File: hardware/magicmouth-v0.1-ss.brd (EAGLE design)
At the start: 100 x 80 mm, 34 parts, among them IC1 LM386N, IC2 ATMEGA328P_PDIP, Q1 16Mhz, U1 ARDUINOR3-NOIOREF-NOTEXT

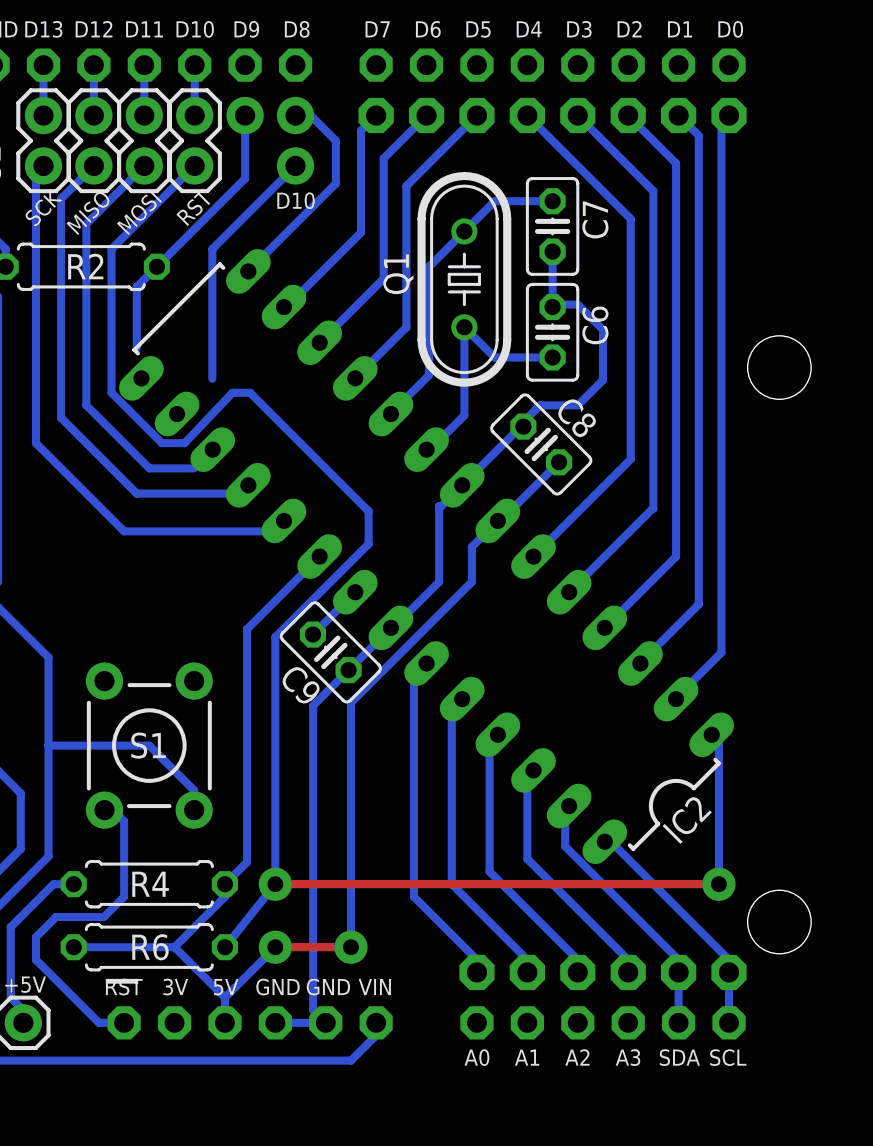
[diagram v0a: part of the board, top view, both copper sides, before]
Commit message: trace corrections
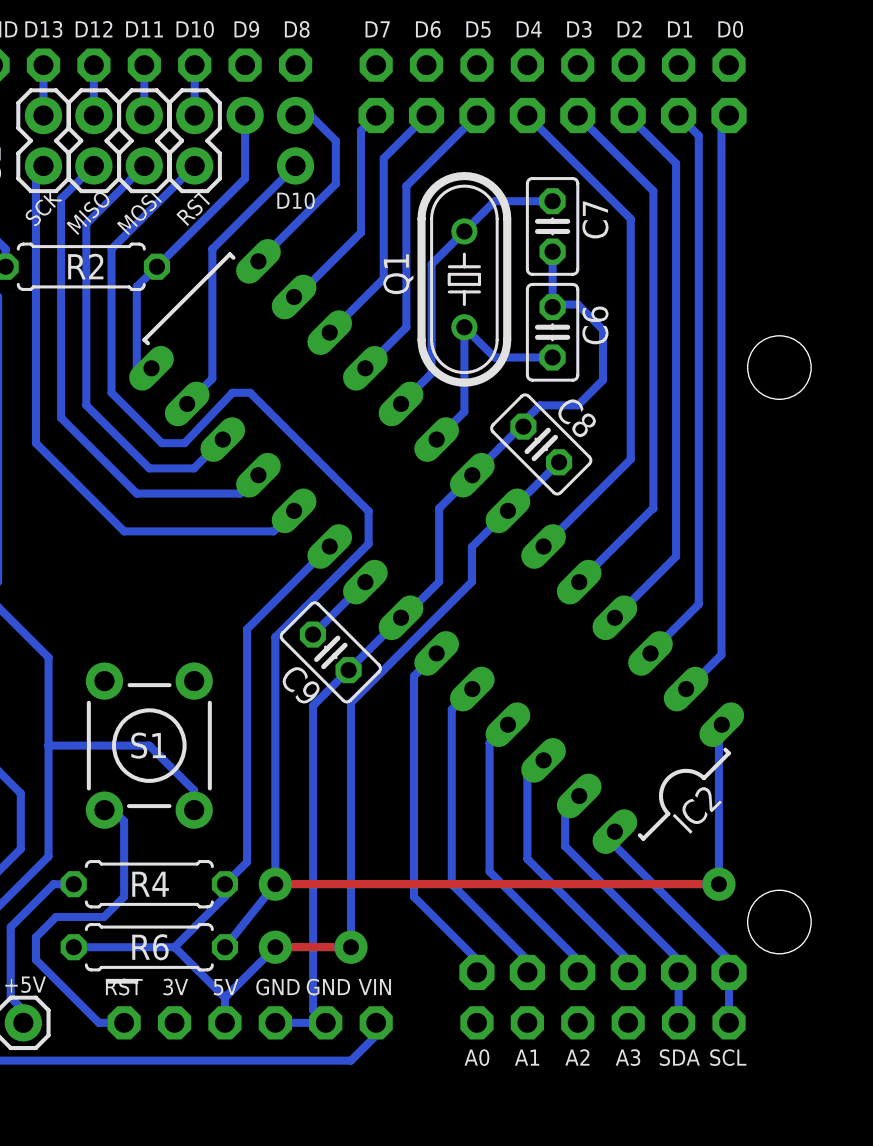
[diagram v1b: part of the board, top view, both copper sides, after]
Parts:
- moved IC2 0.72 mm to (58.9, 36.7)
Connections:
- net MOSI: now also IC2.17
- net N$11: now also IC2.10
- net N$12: now also IC2.16
- net N$13: now also IC2.23
- net N$31: now also IC2.28
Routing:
- net SIGNAL: track 14.0 -> 16.1 mm
- net MOSI: track 20.0 -> 22.1 mm
- net N$12: track 12.5 -> 14.3 mm
- net N$18: track 27.4 -> 29.0 mm
- net N$17: track 28.3 -> 29.9 mm
- net N$13: track 16.3 -> 17.9 mm
- net N$16: track 29.6 -> 30.6 mm
- net N$21: track 15.8 -> 15.1 mm
- net N$34: track 3.01 -> 3.73 mm
- net N$22: track 13.7 -> 13.0 mm
- net N$20: track 26.4 -> 25.7 mm
- net N$19: track 27.4 -> 26.7 mm
- net N$15: track 14.0 -> 14.7 mm
- net MISO: track 24.6 -> 25.3 mm
- net +5V: track 68.9 -> 69.6 mm
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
